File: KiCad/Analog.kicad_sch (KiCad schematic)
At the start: 37 parts, among them J201 OUT+, J202 OUT-, J203 V+, J204 V-, Q201 IRF510, U201 ADR441, U202 LTC1595, U203 OPA4182, U204 AD7789, U205 ORNTA1001AT1

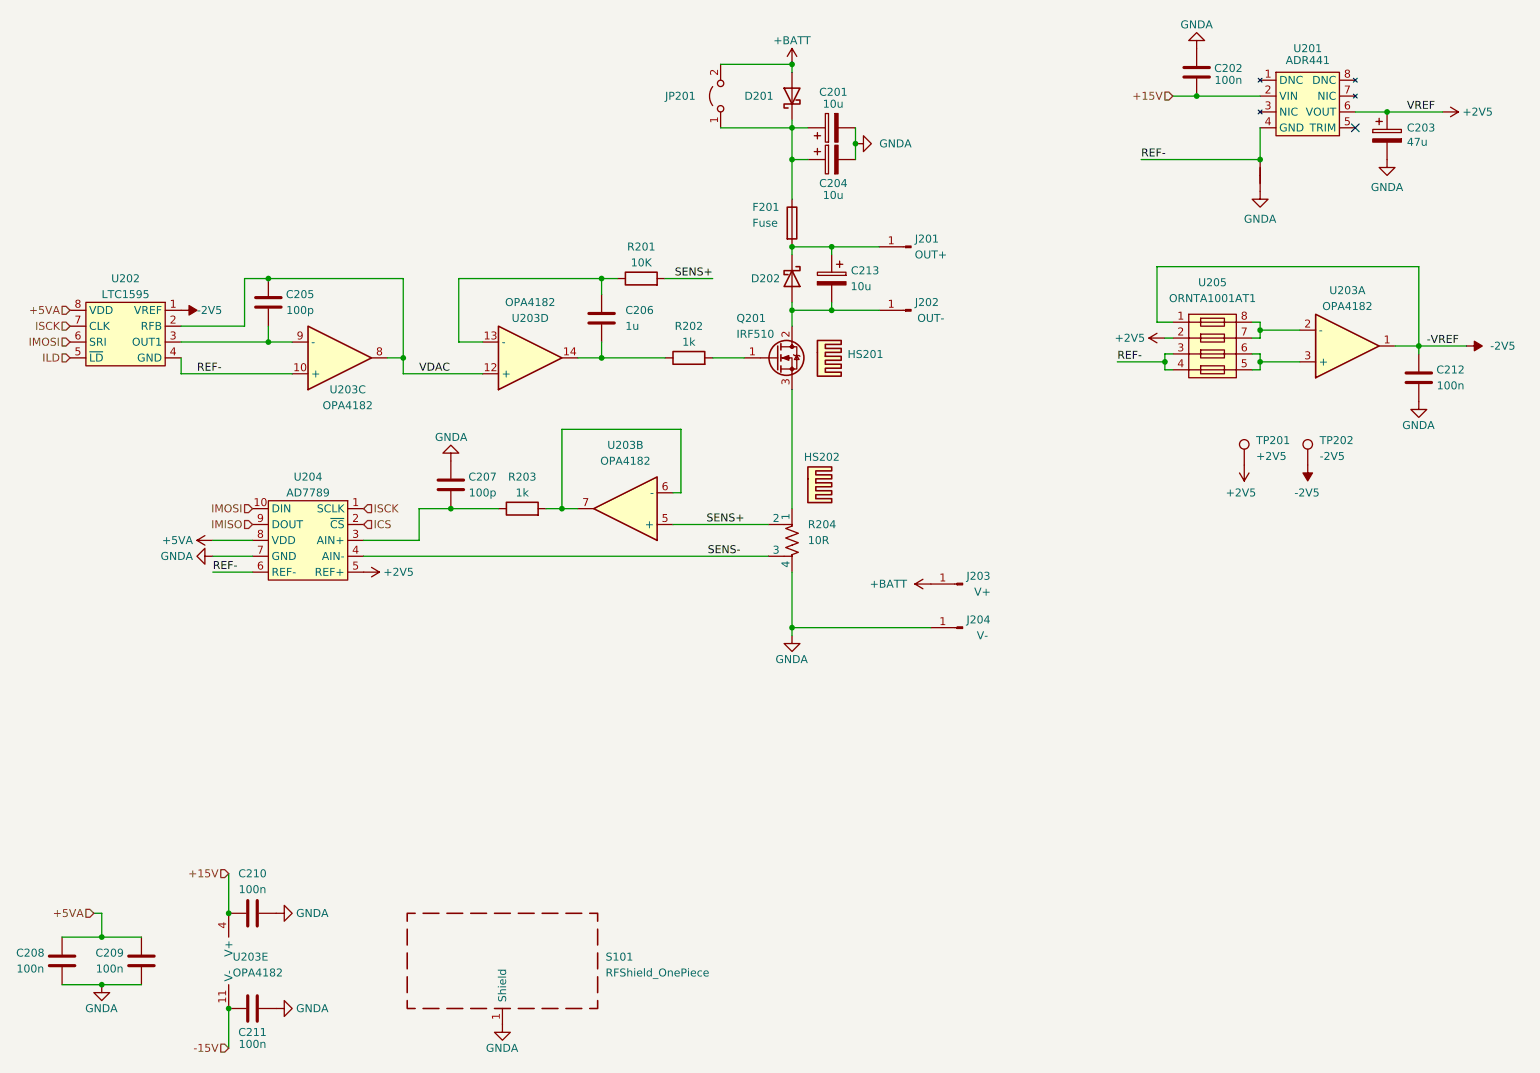
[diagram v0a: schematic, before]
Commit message: Cleaned up a few things
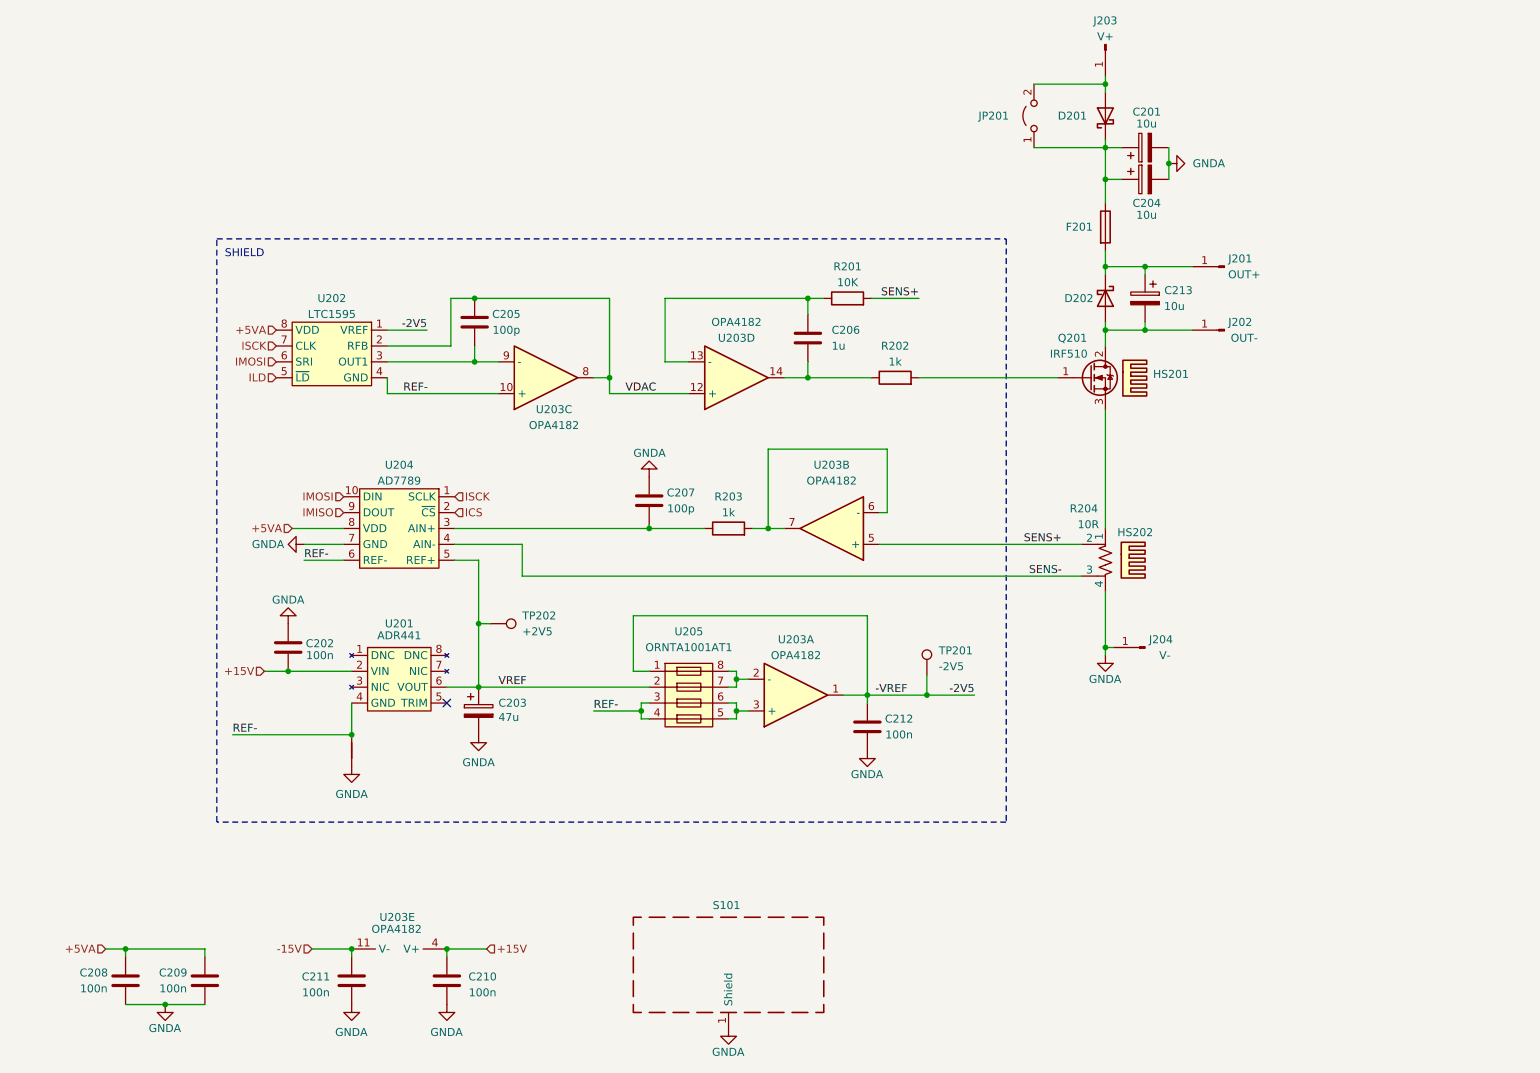
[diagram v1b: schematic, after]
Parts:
- TP201: value +2V5 -> -2V5
- TP202: value -2V5 -> +2V5
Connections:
- net -2V5: now also TP201.1; no longer TP202.1
- net +2V5 renamed VREF
- net VREF: now also TP202.1; no longer TP201.1
- net +BATT: no longer names the net of D201.2 (A), J203.1 (Pin_1), JP201.2 (B)
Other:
- note added: "SHIELD"
- moved on the sheet: C201, C202, C203, C204, C205, C206, C207, C208, C209, C210, C211, C212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
